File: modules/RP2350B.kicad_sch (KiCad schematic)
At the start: 52 parts, among them SW1 SW_Push, SW3 SW_Push, SW4 SW_Push, U1 RP2350B, U5 W25Q128JVS, Y1 12MHz

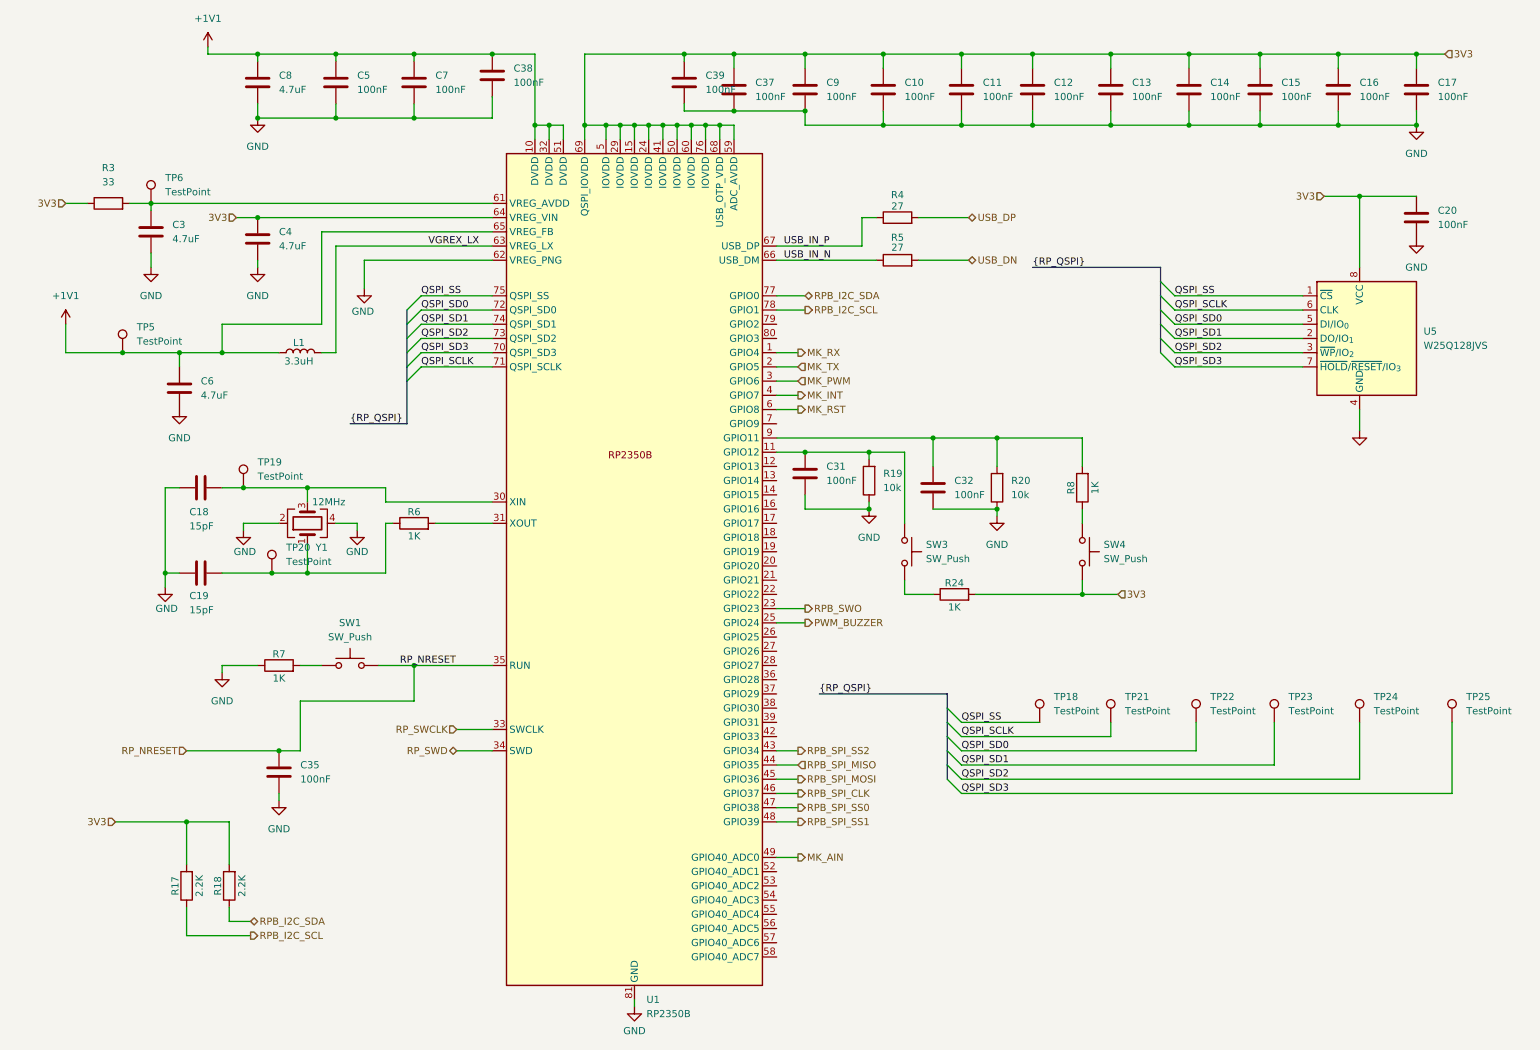
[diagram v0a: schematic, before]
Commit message: Cambio de layout, correccion de pinout
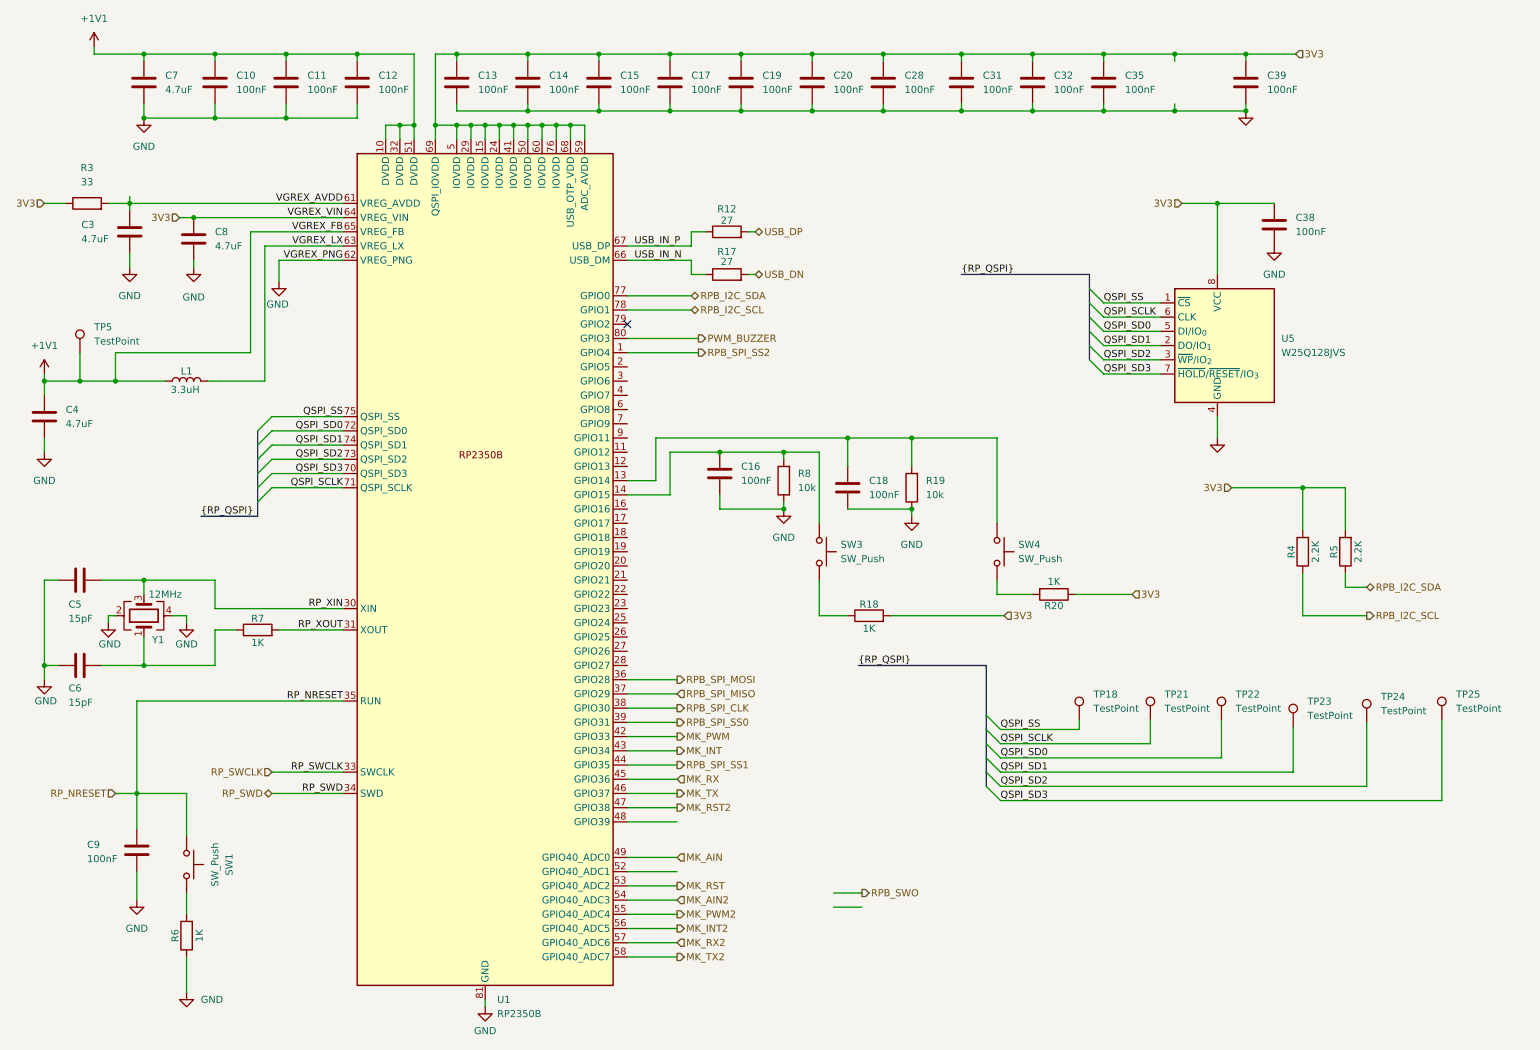
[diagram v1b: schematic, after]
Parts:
- removed C17, C32: 100nF, Capacitor_SMD:C_0402_1005Metric, symbol Device:C
- removed TP19, TP20: TestPoint, TestPoint:TestPoint_Pad_D1.0mm, symbol Connector:TestPoint
- removed TP6: TestPoint, TestPoint:TestPoint_THTPad_D1.0mm_Drill0.5mm, symbol Connector:TestPoint
- added C18: 100nF, Capacitor_SMD:C_0603_1608Metric, symbol Device:C
- added C39: 100nF, Capacitor_SMD:C_0402_1005Metric, symbol Device:C
- C16: renamed from C31; footprint Capacitor_SMD:C_0402_1005Metric -> Capacitor_SMD:C_0603_1608Metric
- C38: renamed from C20; footprint Capacitor_SMD:C_0402_1005Metric -> Capacitor_SMD:C_0603_1608Metric
- C9: renamed from C35; footprint Capacitor_SMD:C_0402_1005Metric -> Capacitor_SMD:C_0603_1608Metric
- R18: renamed from R24; footprint Resistor_SMD:R_0402_1005Metric -> Resistor_SMD:R_0603_1608Metric
- R20: renamed from R8; footprint Resistor_SMD:R_0402_1005Metric -> Capacitor_SMD:C_0603_1608Metric
- R6: renamed from R7; footprint Resistor_SMD:R_0402_1005Metric -> Resistor_SMD:R_0603_1608Metric
- TP18, TP21, TP22, TP23, TP24, TP25: footprint TestPoint:TestPoint_THTPad_D1.0mm_Drill0.5mm -> Sadman_TP:TP_2.8mm_1mm
- TP5: footprint TestPoint:TestPoint_THTPad_D1.5mm_Drill0.7mm -> Sadman_TP:TP_2.8mm_1mm
- renumbered C5 to C10, C7 to C11, C38 to C12, C39 to C13, C37 to C14, C9 to C15, C10 to C17, C11 to C19, C12 to C20, C13 to C28, C14 to C31, C15 to C32, C16 to C35, C6 to C4, C18 to C5, C19 to C6, C8 to C7, C4 to C8, R4 to R12, R5 to R17, R20 to R19, R17 to R4, R18 to R5, R6 to R7, R19 to R8
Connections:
- net 3V3: now also R20.1, C39.1; no longer SW4.2
- net GND: now also C18.2, C39.2
- net MK_INT: now also U1.43 (GPIO34); no longer U1.4 (GPIO7)
- net MK_PWM: now also U1.42 (GPIO33); no longer U1.3 (GPIO6)
- net MK_RST: now also U1.53 (GPIO40_ADC2); no longer U1.6 (GPIO8)
- net MK_RX: now also U1.45 (GPIO36); no longer U1.1 (GPIO4)
- net MK_TX: now also U1.46 (GPIO37); no longer U1.2 (GPIO5)
- net PWM_BUZZER: now also U1.80 (GPIO3); no longer U1.25 (GPIO24)
- net RPB_SPI_CLK: now also U1.38 (GPIO30); no longer U1.46 (GPIO37)
- net RPB_SPI_MISO: now also U1.37 (GPIO29); no longer U1.44 (GPIO35)
- net RPB_SPI_MOSI: now also U1.36 (GPIO28); no longer U1.45 (GPIO36)
- net RPB_SPI_SS0: now also U1.39 (GPIO31); no longer U1.47 (GPIO38)
- net RPB_SPI_SS1: now also U1.44 (GPIO35); no longer U1.48 (GPIO39)
- net RPB_SPI_SS2: now also U1.1 (GPIO4); no longer U1.43 (GPIO34)
- net RPB_SWO: no longer U1.23 (GPIO23)
- net at C16.1, R8.2, SW3.1: now also U1.14 (GPIO15); no longer U1.11 (GPIO12)
- net RP_XIN: now reaches C5.1, U1.30 (XIN), Y1.3
- net VGREX_AVDD: now reaches C3.1, R3.2, U1.61 (VREG_AVDD)
- net RP_XOUT: now reaches R7.2, U1.31 (XOUT)
- net at U1.13 (GPIO14): now also R19.2, SW4.1, C18.1
- net MK_AIN2: now reaches U1.54 (GPIO40_ADC3)
- net MK_PWM2: now reaches U1.55 (GPIO40_ADC4)
- net MK_INT2: now reaches U1.56 (GPIO40_ADC5)
- net MK_RX2: now reaches U1.57 (GPIO40_ADC6)
- net MK_TX2: now reaches U1.58 (GPIO40_ADC7)
- new net: R20.2, SW4.2
- new net MK_RST2: U1.47 (GPIO38)
- now unconnected: U1.9 (GPIO11)
- no-connect marks 0 -> 1
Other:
- moved on the sheet: C10, C11, C12, C13, C14, C15, C16, C17, C19, C20, C28, C3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
